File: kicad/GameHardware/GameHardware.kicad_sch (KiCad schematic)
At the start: 9 parts, among them U1 MAX7219, U2 ATmega328P-P, U4 HDSP-7403, U5 HDSP-7403, U6 HDSP-7403, U7 HDSP-7403, U8 HDSP-7403, U9 HDSP-7403

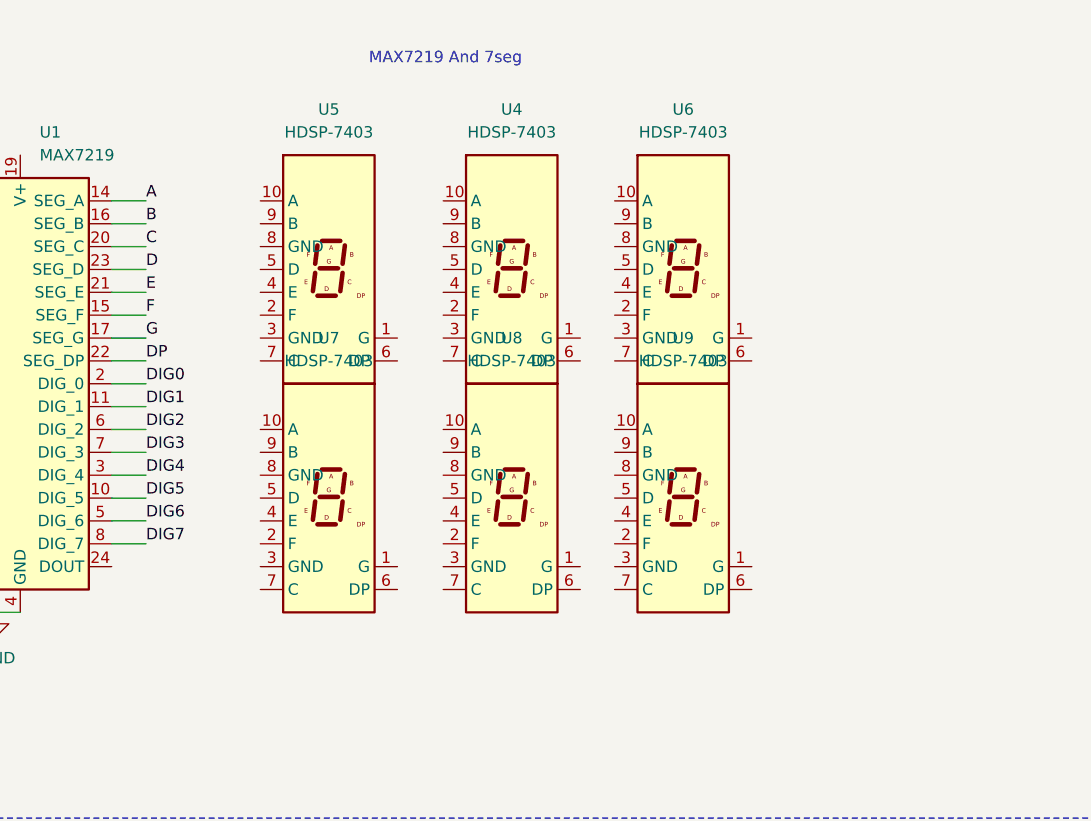
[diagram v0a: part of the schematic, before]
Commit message: pill
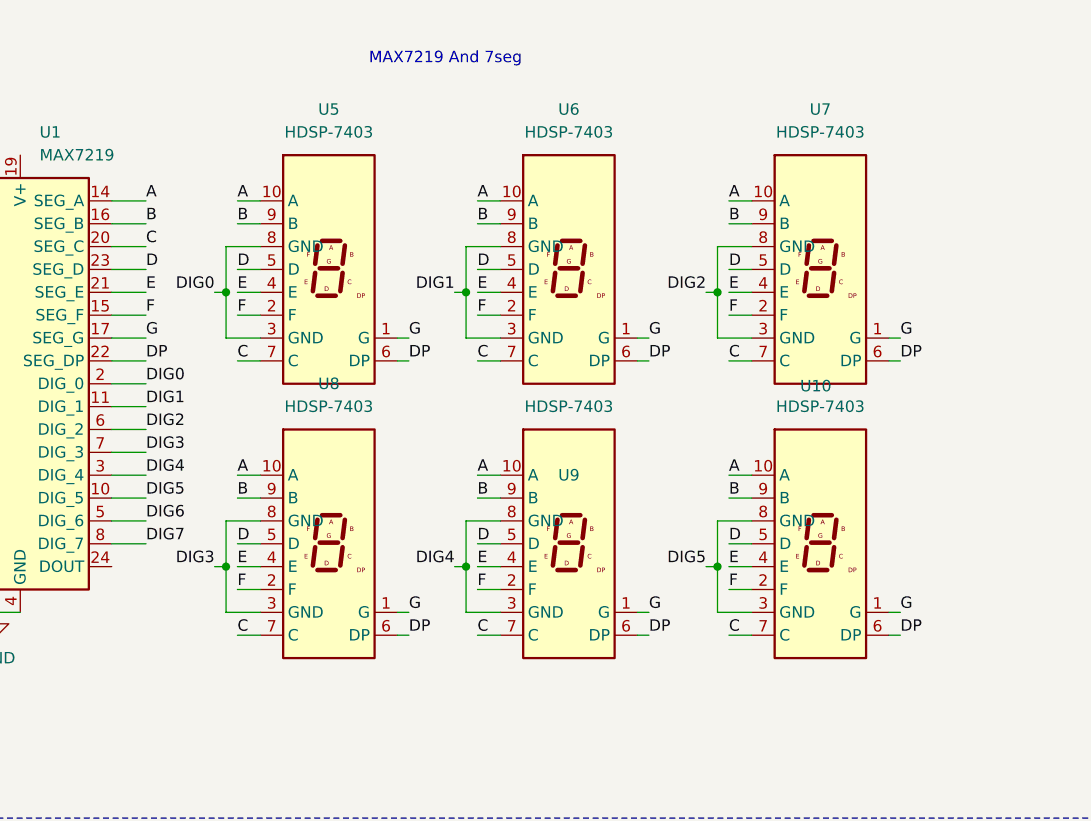
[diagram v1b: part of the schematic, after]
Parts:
- removed U4: HDSP-7403, Display_7Segment:Sx39-1xxxxx, symbol Display_Character:HDSP-7403
- added U10: HDSP-7403, Display_7Segment:Sx39-1xxxxx, symbol Display_Character:HDSP-7403
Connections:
- net A: now also U5.10 (A), U6.10 (A), U7.10 (A), U8.10 (A), U9.10 (A), U10.10 (A)
- net B: now also U5.9 (B), U6.9 (B), U7.9 (B), U8.9 (B), U9.9 (B), U10.9 (B)
- net C: now also U5.7 (C), U6.7 (C), U7.7 (C), U8.7 (C), U9.7 (C), U10.7 (C)
- net D: now also U5.5 (D), U6.5 (D), U7.5 (D), U8.5 (D), U9.5 (D), U10.5 (D)
- net DIG0: now also U5.3 (GND), U5.8 (GND)
- net DIG1: now also U6.3 (GND), U6.8 (GND)
- net DIG2: now also U7.3 (GND), U7.8 (GND)
- net DIG3: now also U8.3 (GND), U8.8 (GND)
- net DIG4: now also U9.3 (GND), U9.8 (GND)
- net DIG5: now also U10.3 (GND), U10.8 (GND)
- net DP: now also U5.6 (DP), U6.6 (DP), U7.6 (DP), U8.6 (DP), U9.6 (DP), U10.6 (DP)
- net E: now also U5.4 (E), U6.4 (E), U7.4 (E), U8.4 (E), U9.4 (E), U10.4 (E)
- net F: now also U5.2 (F), U6.2 (F), U7.2 (F), U8.2 (F), U9.2 (F), U10.2 (F)
- net G: now also U5.1 (G), U6.1 (G), U7.1 (G), U8.1 (G), U9.1 (G), U10.1 (G)
